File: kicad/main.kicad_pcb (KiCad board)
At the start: 2 copper layers, 12 parts, among them J1 Conn_02x14_Counter_Clockwise, U1 7421, U2 74LS86, U3 74LS138, U4 7421, U5 7421, U6 74LS138

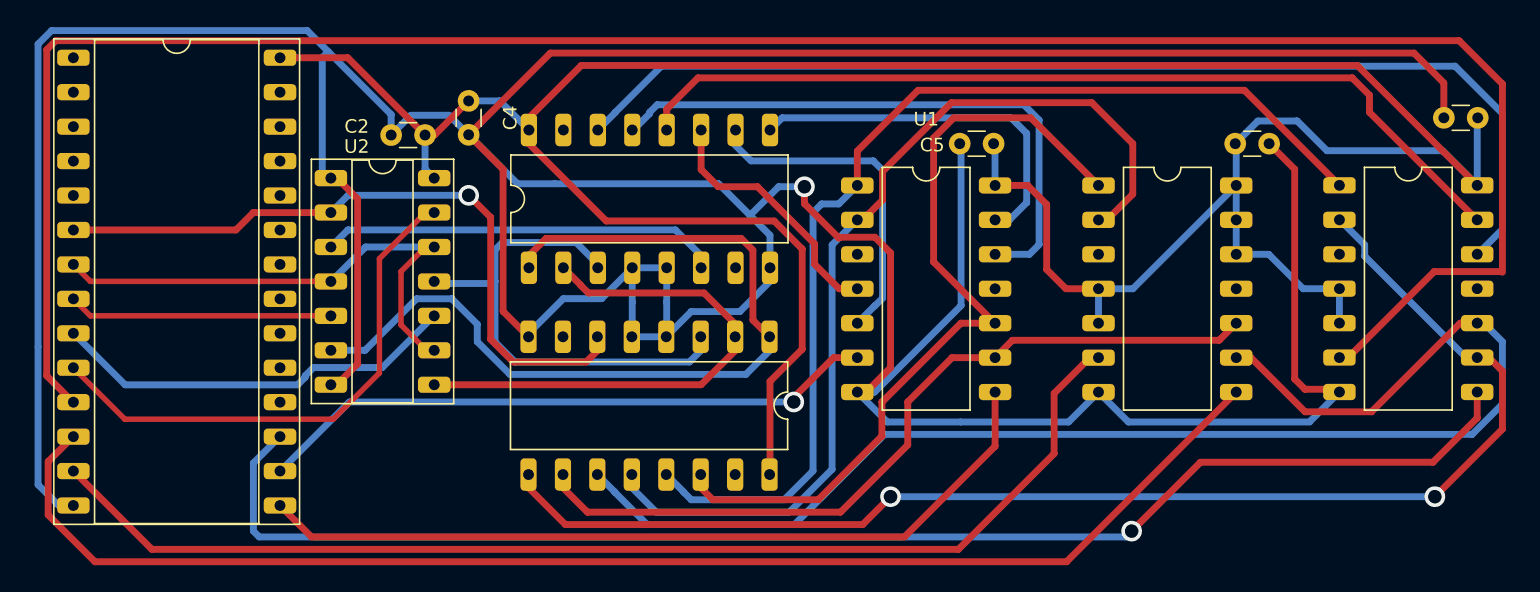
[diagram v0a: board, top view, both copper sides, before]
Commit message: final design
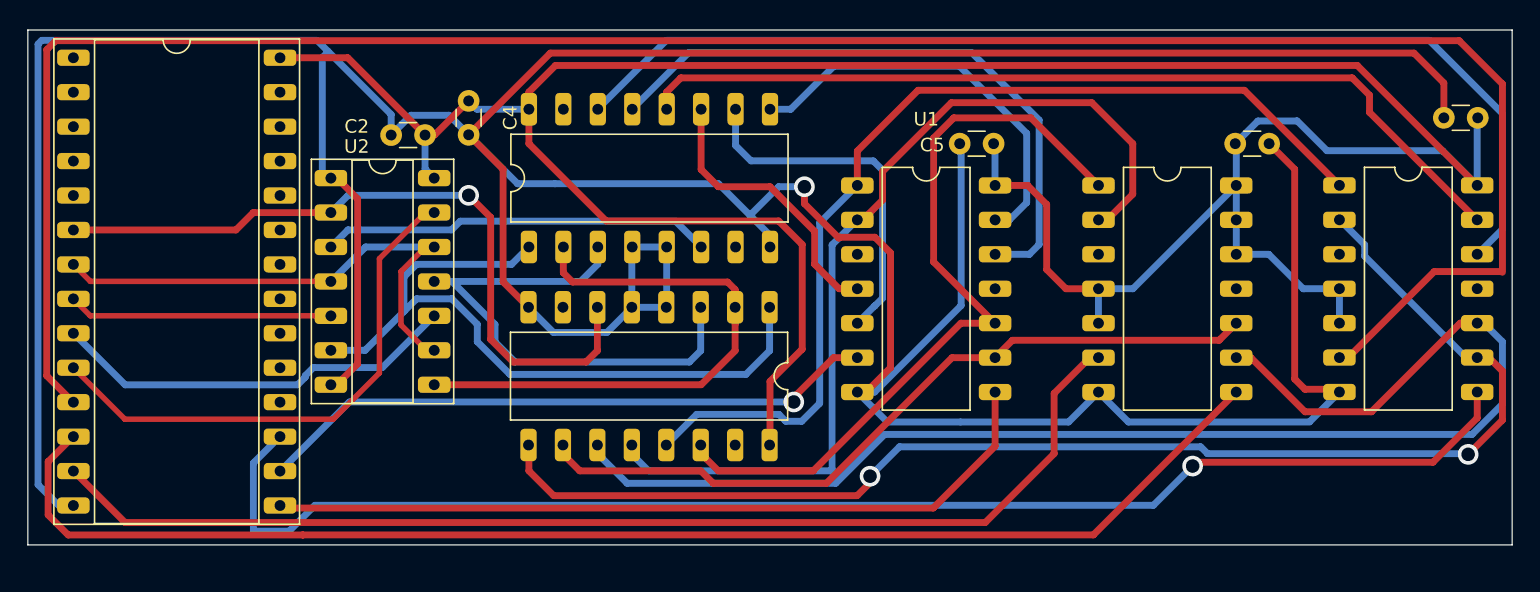
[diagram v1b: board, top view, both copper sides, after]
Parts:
- moved U6 2.18 mm to (101.6, 80.6)
- moved U3 1.53 mm to (83.8, 76.2)
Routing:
- net GND: track 367.8 -> 351.2 mm
- net /adressInverter/H1_OUT: track 64.0 -> 54.3 mm
- net Net-(U6-~{Y2}): track 78.5 -> 73.1 mm
- net /adressInverter/H2_OUT: track 40.4 -> 44.1 mm
- net /adressInverter/H3_OUT: track 37.4 -> 40.5 mm
- net Net-(U6-~{Y5}): track 59.0 -> 56.1 mm
- net Net-(U3-~{Y2}): track 44.0 -> 46.6 mm
- net Net-(U3-~{Y6}): track 27.7 -> 30.3 mm
- net Net-(U6-~{Y1}): track 60.4 -> 57.9 mm
- net Net-(U3-~{Y4}): track 19.0 -> 21.0 mm
- net Net-(U6-~{Y3}): track 71.3 -> 69.5 mm
- net /PWM_IN: track 51.2 -> 53.0 mm
- net /B_L_OUT: track 60.5 -> 58.7 mm
- net /G_H_OUT: track 100.8 -> 99.2 mm
- net /Y_H_OUT: track 86.5 -> 84.8 mm
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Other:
- board outline added: 109.5 x 38 mm
